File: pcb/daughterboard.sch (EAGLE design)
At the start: 21 parts, among them IC3 STM32F042F4, SW1 324_SW324_SWITCH_FOOT_HOLE, SW2 324_SW324_SWITCH_FOOT_HOLE, SW3 324_SW, SW4 324_SW, SW5 324_SW324_SWITCH_FOOT_HOLE, SW6 324_SW324_SWITCH_FOOT_HOLE, U2 USBC_16P, U4 XC6206_DEV

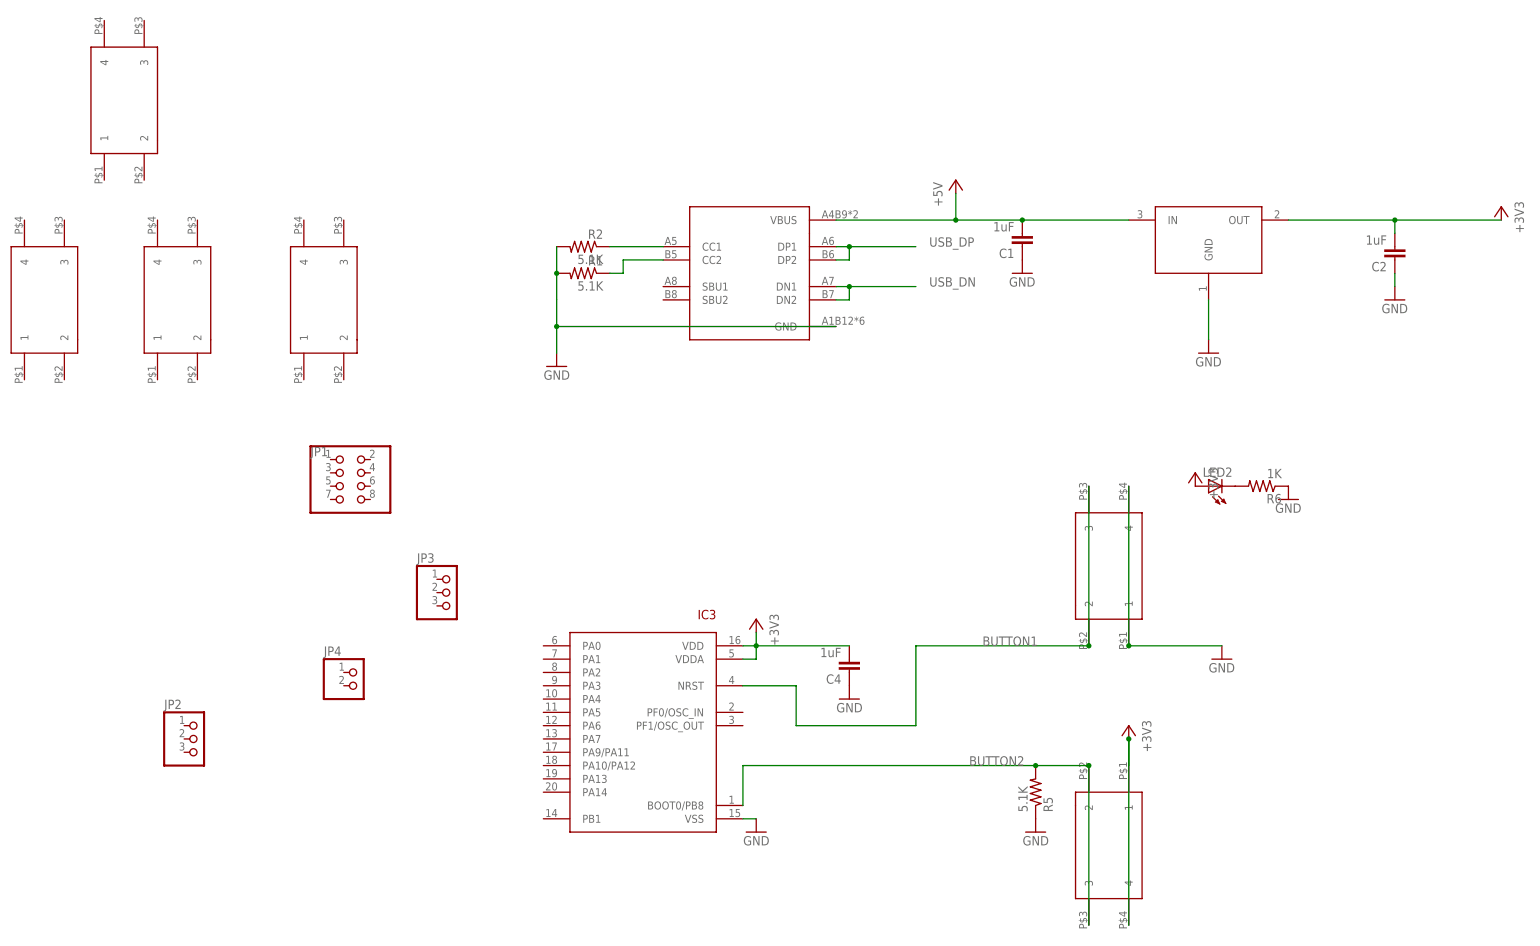
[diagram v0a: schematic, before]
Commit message: working on new version
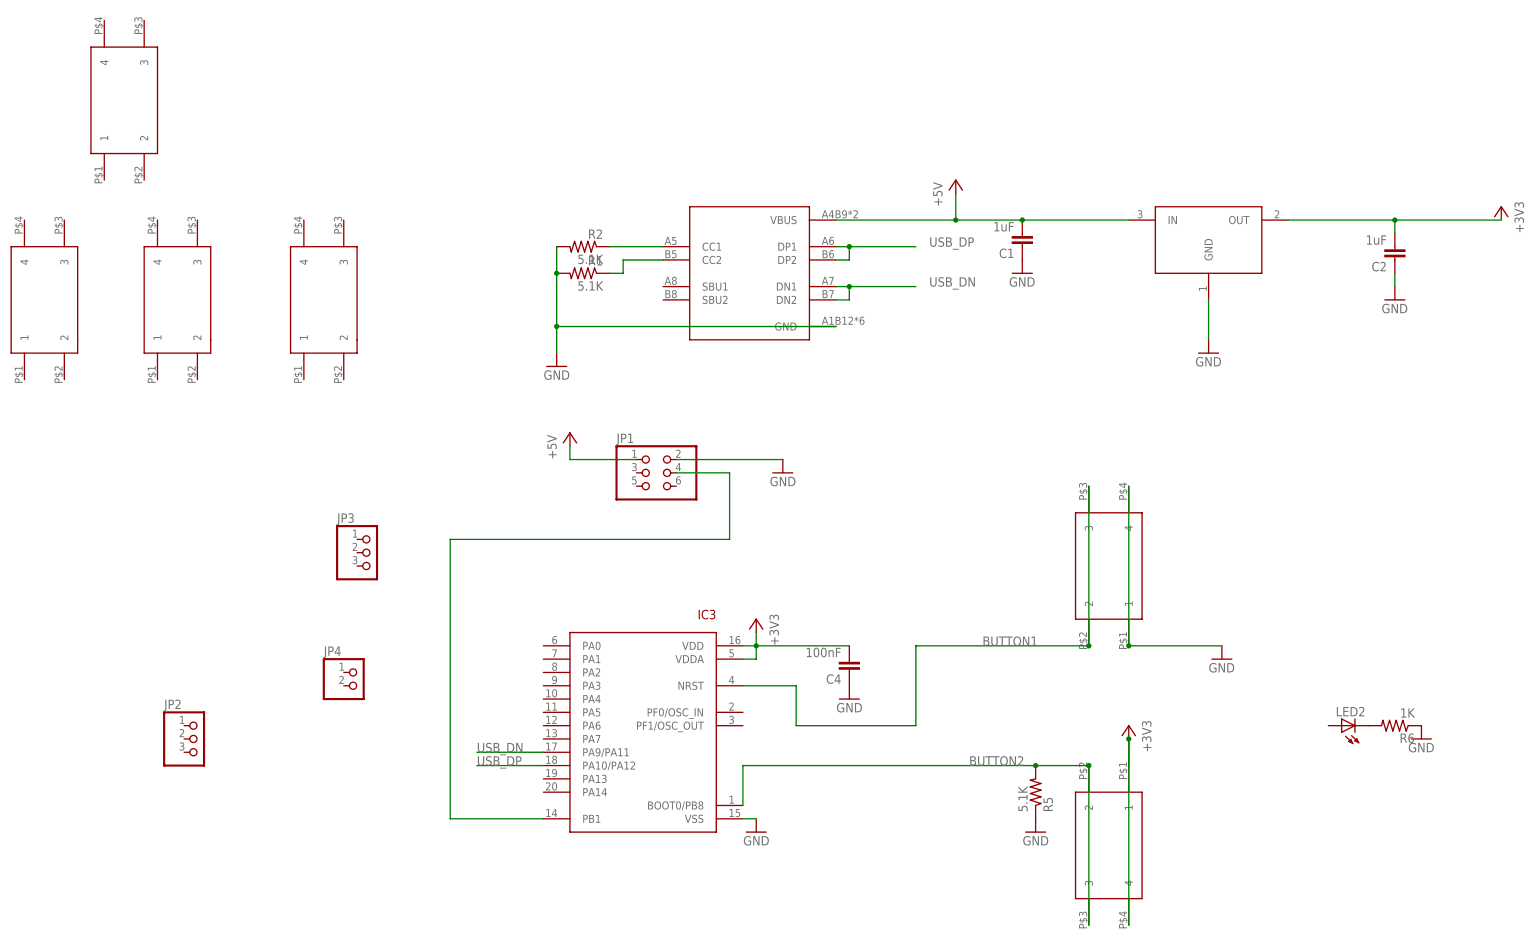
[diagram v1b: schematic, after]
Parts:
- C4: value 1uF -> 100nF
- JP1: device pinhead:PINHD-2X4 -> pinhead:PINHD-2X3
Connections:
- new net N$1: IC3.PB1, JP1.4
- net +3V3: no longer LED2.A
- net +5V: now also JP1.1
- net GND: now also JP1.2
- net USB_DN: now also IC3.PA9/PA11
- net USB_DP: now also IC3.PA10/PA12
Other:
- moved on the sheet: JP3, LED2, R6
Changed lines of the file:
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@@
 <part name="+3V1" library="supply1" library_urn="urn:adsk.eagle:library:371" deviceset="+3V3" device=""/>
 <part name="GND5" library="supply1" deviceset="GND" device=""/>
-<part name="C4" library="clock" deviceset="CAP" device="0805" value="1uF"/>
+<part name="C4" library="clock" deviceset="CAP" device="0805" value="100nF"/>
 <part name="GND8" library="supply1" deviceset="GND" device=""/>
 <part name="GND11" library="supply1" library_urn="urn:adsk.eagle:library:371" deviceset="GND" device=""/>
 <part name="SW3" library="3pos_slide_switch_centered" deviceset="324_SW" device="" value="324_SW"/>
 <part name="SW4" library="3pos_slide_switch_centered" deviceset="324_SW" device="" value="324_SW"/>
-<part name="+3V16" library="backplane" deviceset="+3V3" device=""/>
 <part name="LED2" library="adafruit" deviceset="LED" device="CHIP-LED0805"/>
 <part name="R6" library="SparkFun-Passives" deviceset="RESISTOR" device="0805-RES" value="1K"/>
@@
 <part name="U4" library="3pos_slide_switch" deviceset="XC6206_DEV" device=""/>
 <part name="C2" library="clock" deviceset="CAP" device="0805" value="1uF"/>
-<part name="JP1" library="pinhead" library_urn="urn:adsk.eagle:library:325" deviceset="PINHD-2X4" device="" package3d_urn="urn:adsk.eagle:package:22461/2"/>
+<part name="JP1" library="pinhead" library_urn="urn:adsk.eagle:library:325" deviceset="PINHD-2X3" device="" package3d_urn="urn:adsk.eagle:package:22462/2"/>
 <part name="SW2" library="3pos_slide_switch" deviceset="324_SW" device="324_SWITCH_FOOT_HOLE" value="324_SW324_SWITCH_FOOT_HOLE"/>
 <part name="SW1" library="3pos_slide_switch" deviceset="324_SW" device="324_SWITCH_FOOT_HOLE" value="324_SW324_SWITCH_FOOT_HOLE"/>
@@
 <part name="JP3" library="pinhead" library_urn="urn:adsk.eagle:library:325" deviceset="PINHD-1X3" device="" package3d_urn="urn:adsk.eagle:package:22458/2"/>
 <part name="JP4" library="pinhead" library_urn="urn:adsk.eagle:library:325" deviceset="PINHD-1X2" device="" package3d_urn="urn:adsk.eagle:package:22435/2"/>
+<part name="P+2" library="supply1" library_urn="urn:adsk.eagle:library:371" deviceset="+5V" device=""/>
+<part name="GND2" library="supply1" deviceset="GND" device=""/>
 </parts>
 <sheets>
@@
 <instance part="SW3" gate="G$1" x="91.44" y="55.88" smashed="yes" rot="R90"/>
 <instance part="SW4" gate="G$1" x="91.44" y="2.54" smashed="yes" rot="MR270"/>
-<instance part="+3V16" gate="G$1" x="106.68" y="73.66" smashed="yes" rot="MR0">
-<attribute name="VALUE" x="109.22" y="68.58" size="1.778" layer="96" rot="MR90"/>
-</instance>
-<instance part="LED2" gate="G$1" x="109.22" y="71.12" smashed="yes" rot="R90">
-<attribute name="NAME" x="113.792" y="74.676" size="1.778" layer="95" rot="R180"/>
-<attribute name="VALUE" x="113.792" y="76.835" size="1.778" layer="96" rot="R180"/>
-</instance>
-<instance part="R6" gate="G$1" x="119.38" y="71.12" smashed="yes" rot="R180">
-<attribute name="NAME" x="123.19" y="69.6214" size="1.778" layer="95" rot="R180"/>
-<attribute name="VALUE" x="123.19" y="74.422" size="1.778" layer="96" rot="R180"/>
-</instance>
-<instance part="GND9" gate="1" x="124.46" y="68.58" smashed="yes">
-<attribute name="VALUE" x="121.92" y="66.04" size="1.778" layer="96"/>
+<instance part="LED2" gate="G$1" x="134.62" y="25.4" smashed="yes" rot="R90">
+<attribute name="NAME" x="139.192" y="28.956" size="1.778" layer="95" rot="R180"/>
+<attribute name="VALUE" x="139.192" y="31.115" size="1.778" layer="96" rot="R180"/>
+</instance>
+<instance part="R6" gate="G$1" x="144.78" y="25.4" smashed="yes" rot="R180">
+<attribute name="NAME" x="148.59" y="23.9014" size="1.778" layer="95" rot="R180"/>
+<attribute name="VALUE" x="148.59" y="28.702" size="1.778" layer="96" rot="R180"/>
+</instance>
+<instance part="GND9" gate="1" x="149.86" y="22.86" smashed="yes">
+<attribute name="VALUE" x="147.32" y="20.32" size="1.778" layer="96"/>
 </instance>
 <instance part="+3V2" gate="G$1" x="93.98" y="25.4" smashed="yes" rot="MR0">
@@
 <attribute name="VALUE" x="143.256" y="118.999" size="1.778" layer="96" rot="R180"/>
 </instance>
-<instance part="JP1" gate="A" x="-55.88" y="71.12" smashed="yes">
-<attribute name="NAME" x="-62.23" y="76.835" size="1.778" layer="95"/>
-<attribute name="VALUE" x="-62.23" y="63.5" size="1.778" layer="96"/>
+<instance part="JP1" gate="A" x="2.54" y="73.66" smashed="yes">
+<attribute name="NAME" x="-3.81" y="79.375" size="1.778" layer="95"/>
+<attribute name="VALUE" x="-3.81" y="66.04" size="1.778" layer="96"/>
 </instance>
 <instance part="SW2" gate="G$1" x="-60.96" y="106.68" smashed="yes" rot="MR90"/>
@@
 <attribute name="VALUE" x="-90.17" y="15.24" size="1.778" layer="96"/>
 </instance>
-<instance part="JP3" gate="A" x="-35.56" y="50.8" smashed="yes">
-<attribute name="NAME" x="-41.91" y="56.515" size="1.778" layer="95"/>
-<attribute name="VALUE" x="-41.91" y="43.18" size="1.778" layer="96"/>
+<instance part="JP3" gate="A" x="-50.8" y="58.42" smashed="yes">
+<attribute name="NAME" x="-57.15" y="64.135" size="1.778" layer="95"/>
+<attribute name="VALUE" x="-57.15" y="50.8" size="1.778" layer="96"/>
 </instance>
 <instance part="JP4" gate="G$1" x="-53.34" y="33.02" smashed="yes">
 <attribute name="NAME" x="-59.69" y="38.735" size="1.778" layer="95"/>
 <attribute name="VALUE" x="-59.69" y="27.94" size="1.778" layer="96"/>
+</instance>
+<instance part="P+2" gate="1" x="-12.7" y="81.28" smashed="yes">
+<attribute name="VALUE" x="-15.24" y="76.2" size="1.778" layer="96" rot="R90"/>
+</instance>
+<instance part="GND2" gate="1" x="27.94" y="73.66" smashed="yes" rot="MR0">
+<attribute name="VALUE" x="30.48" y="71.12" size="1.778" layer="96" rot="MR0"/>
 </instance>
 </instances>
@@
 <wire x1="144.78" y1="111.76" x2="144.78" y2="109.22" width="0.1524" layer="91"/>
 </segment>
+<segment>
+<pinref part="JP1" gate="A" pin="2"/>
+<pinref part="GND2" gate="1" pin="GND"/>
+<wire x1="7.62" y1="76.2" x2="27.94" y2="76.2" width="0.1524" layer="91"/>
+</segment>
 </net>
 <net name="+3V3" class="0">
@@
 </segment>
 <segment>
-<pinref part="+3V16" gate="G$1" pin="+3V3"/>
-<pinref part="LED2" gate="G$1" pin="A"/>
-</segment>
-<segment>
 <pinref part="SW4" gate="G$1" pin="1"/>
 <pinref part="SW4" gate="G$1" pin="4"/>
@@
 <wire x1="40.64" y1="114.3" x2="38.1" y2="114.3" width="0.1524" layer="91"/>
 </segment>
+<segment>
+<pinref part="IC3" gate="G$1" pin="PA10/PA12"/>
+<wire x1="-17.78" y1="17.78" x2="-30.48" y2="17.78" width="0.1524" layer="91"/>
+<label x="-30.48" y="17.78" size="1.778" layer="95"/>
+</segment>
 </net>
 <net name="N$31" class="0">
@@
 <wire x1="40.64" y1="106.68" x2="40.64" y2="109.22" width="0.1524" layer="91"/>
 <junction x="40.64" y="109.22"/>
+</segment>
+<segment>
+<pinref part="IC3" gate="G$1" pin="PA9/PA11"/>
+<wire x1="-17.78" y1="20.32" x2="-30.48" y2="20.32" width="0.1524" layer="91"/>
+<label x="-30.48" y="20.32" size="1.778" layer="95"/>
 </segment>
 </net>
@@
 <junction x="60.96" y="121.92"/>
 <pinref part="U4" gate="G$1" pin="IN"/>
+</segment>
+<segment>
+<pinref part="JP1" gate="A" pin="1"/>
+<pinref part="P+2" gate="1" pin="+5V"/>
+<wire x1="0" y1="76.2" x2="-12.7" y2="76.2" width="0.1524" layer="91"/>
+<wire x1="-12.7" y1="76.2" x2="-12.7" y2="78.74" width="0.1524" layer="91"/>
 </segment>
 </net>
@@
 </segment>
 </net>
+<net name="N$1" class="0">
+<segment>
+<pinref part="IC3" gate="G$1" pin="PB1"/>
+<wire x1="-17.78" y1="7.62" x2="-35.56" y2="7.62" width="0.1524" layer="91"/>
+<wire x1="-35.56" y1="7.62" x2="-35.56" y2="60.96" width="0.1524" layer="91"/>
+<wire x1="-35.56" y1="60.96" x2="17.78" y2="60.96" width="0.1524" layer="91"/>
+<wire x1="17.78" y1="60.96" x2="17.78" y2="73.66" width="0.1524" layer="91"/>
+<pinref part="JP1" gate="A" pin="4"/>
+<wire x1="17.78" y1="73.66" x2="7.62" y2="73.66" width="0.1524" layer="91"/>
+</segment>
+</net>
